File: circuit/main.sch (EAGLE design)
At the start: 18 parts, among them IC2 LD398533RM, J1 22-27-2041-04, J2 22-27-2041-04, Q2 BSS138, Q3 12MHz, U1 ATTINY84-20SSU

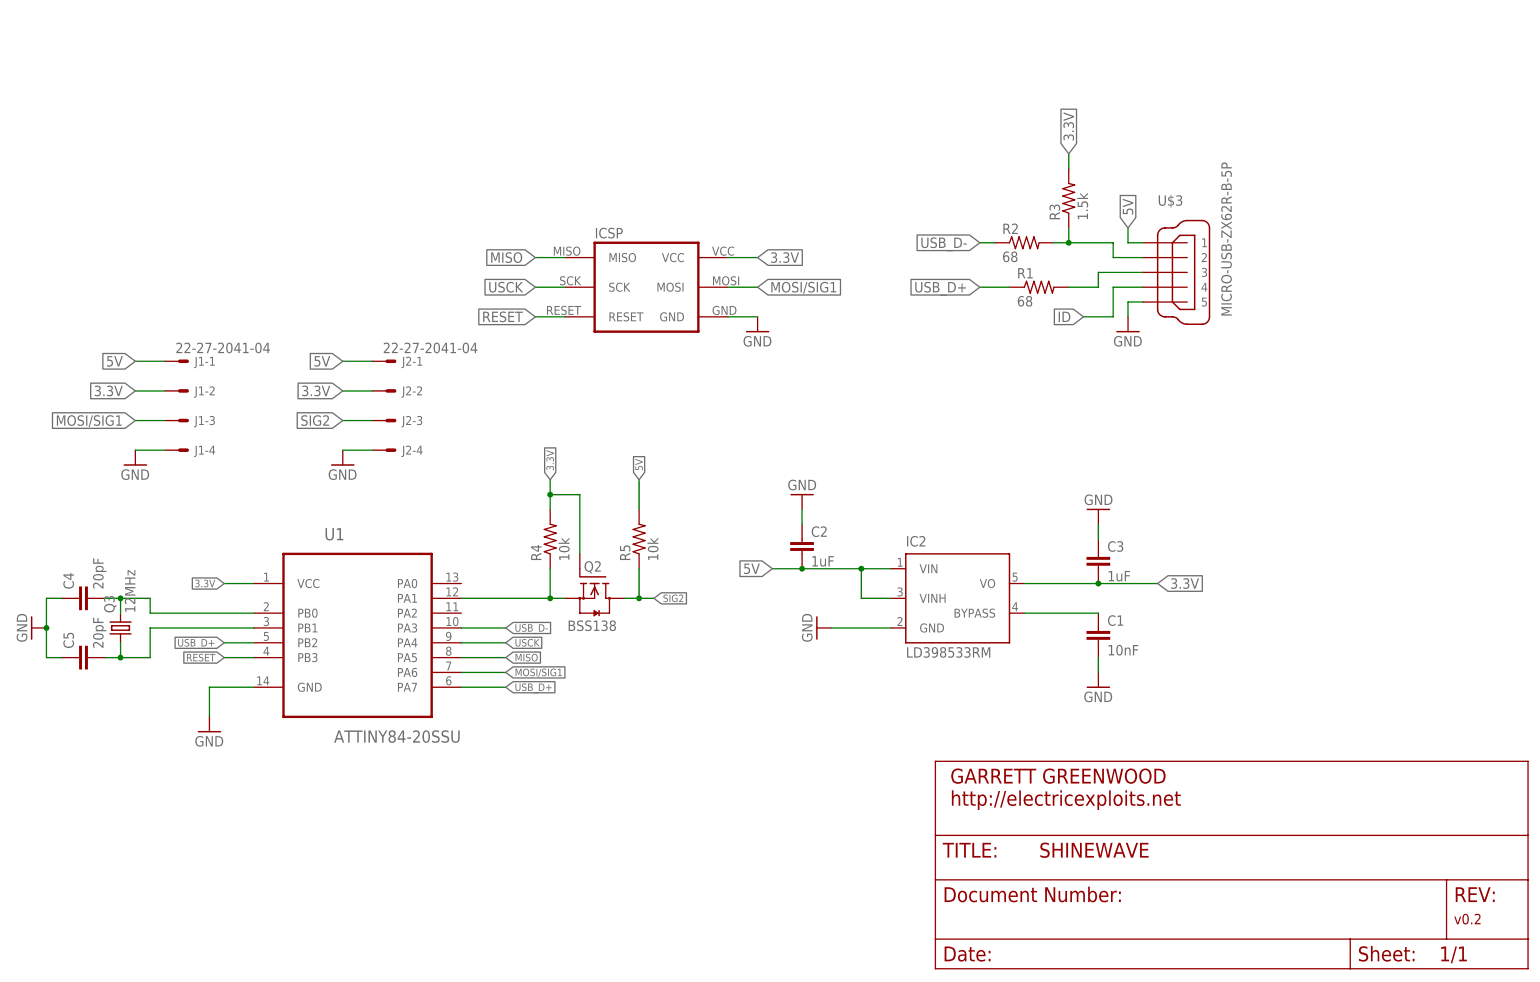
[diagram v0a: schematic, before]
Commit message: my own board
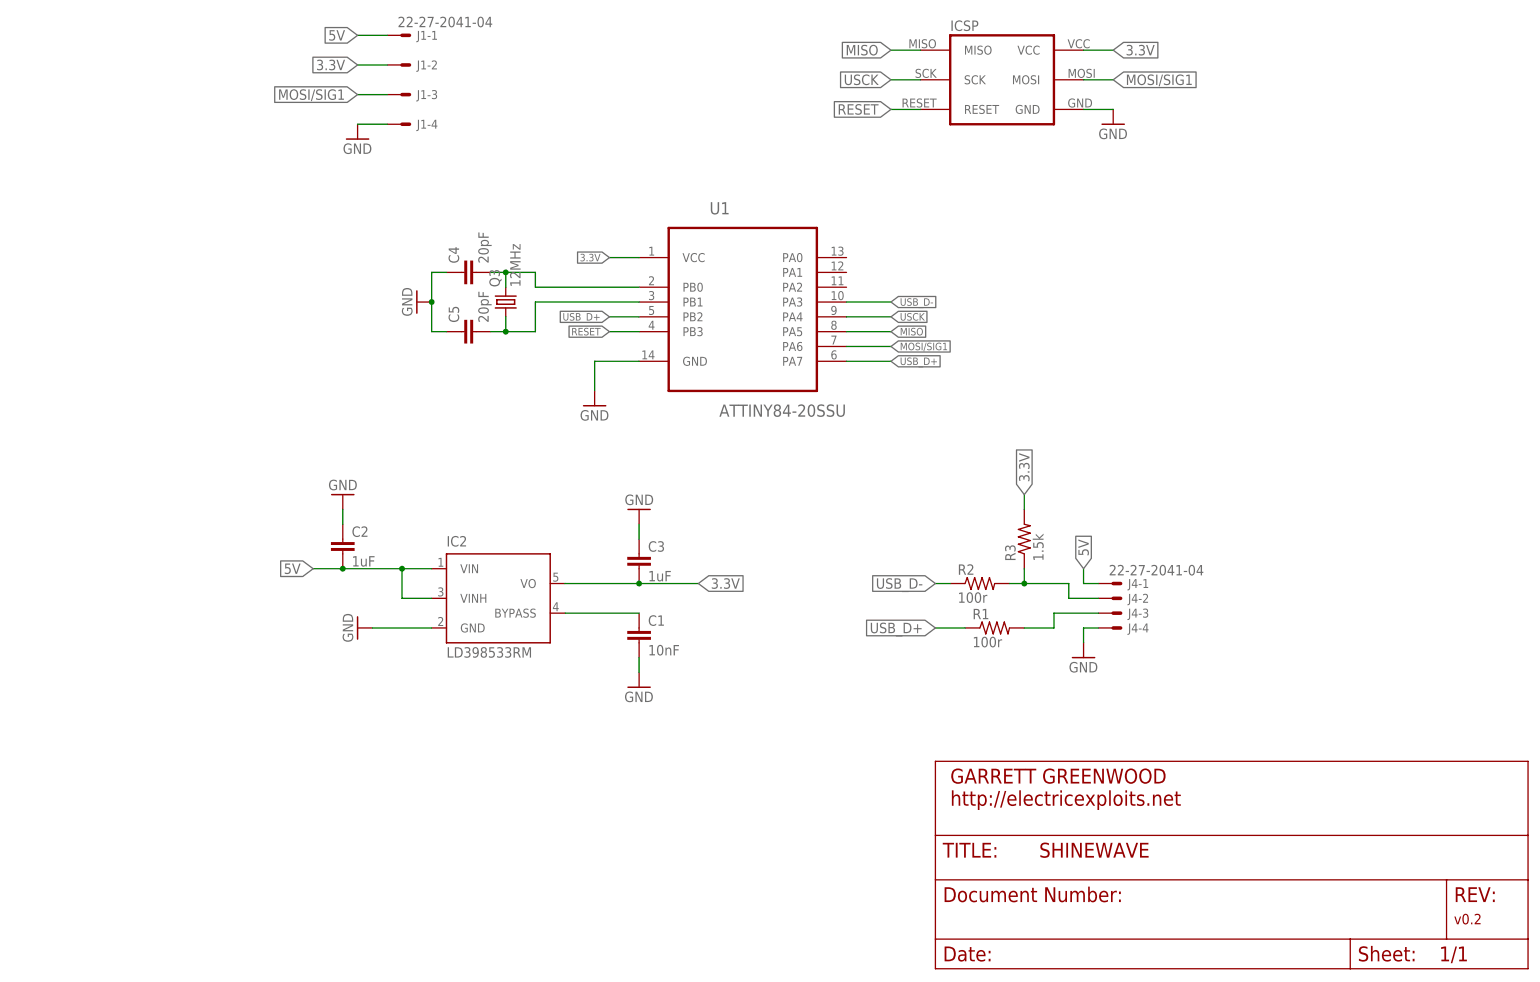
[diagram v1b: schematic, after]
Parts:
- removed J2: 22-27-2041-04, con-molex:22-27-2041-04
- removed Q2: BSS138, m-pad-2.1:BSS138
- removed R4, R5: 10k, resistor:R-US_R0603
- removed U$3: MICRO-USB-ZX62R-B-5P, con-hirose:MICRO-USB-ZX62R-B-5P
- added J4: 22-27-2041-04, con-molex:22-27-2041-04
- R1, R2: value 68 -> 100r
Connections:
- removed net ID: U$3.4
- removed net N$1: Q2.S, R4.1, U1.PA1
- removed net SIG2: J2-3.S, Q2.D, R5.1
- net 3.3V: no longer J2-2.S, Q2.G, R4.2
- net 5V: now also J4-1.S; no longer J2-1.S, R5.2, U$3.1
- net GND: now also J4-4.S; no longer J2-4.S, U$3.5
- net N$2: now also J4-2.S; no longer U$3.2
- net N$5: now also J4-3.S; no longer U$3.3
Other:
- moved on the sheet: C1, C2, C3, C4, C5, IC2, J1-1, J1-2, J1-3, J1-4, Q3, R1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
